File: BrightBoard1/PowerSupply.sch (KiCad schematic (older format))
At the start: 21 parts, among them J2 VIN_JACK, U2 TPS62177DQC

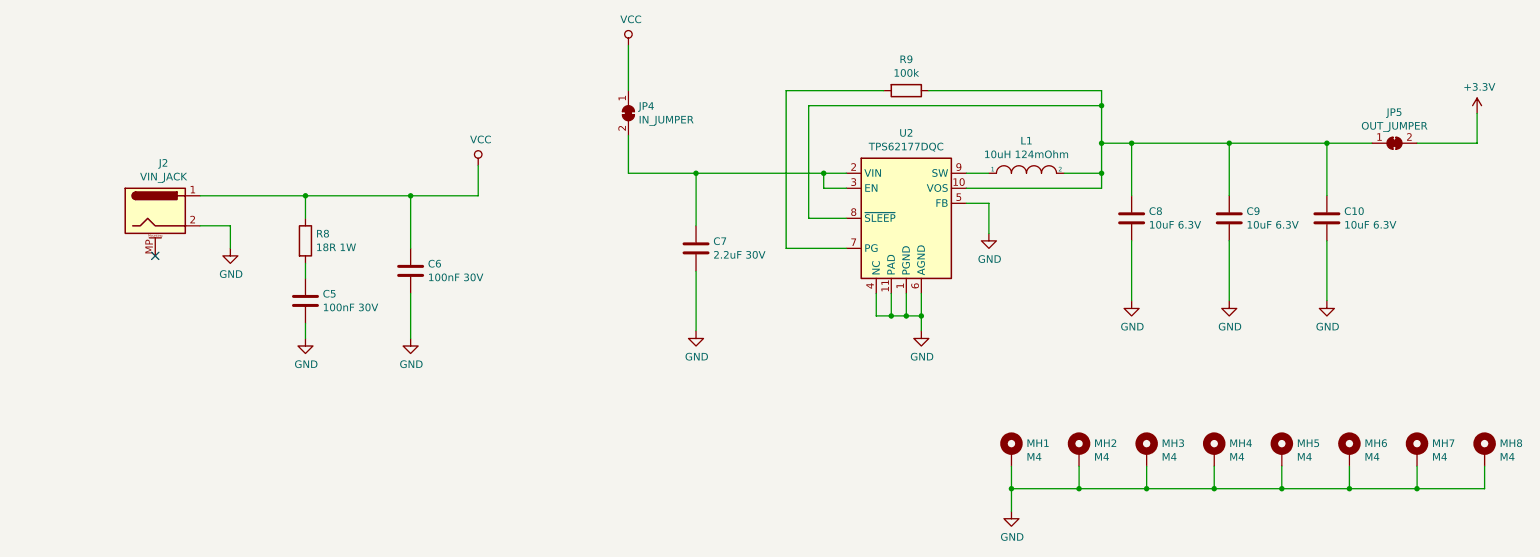
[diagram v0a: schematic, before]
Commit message: Moving over?
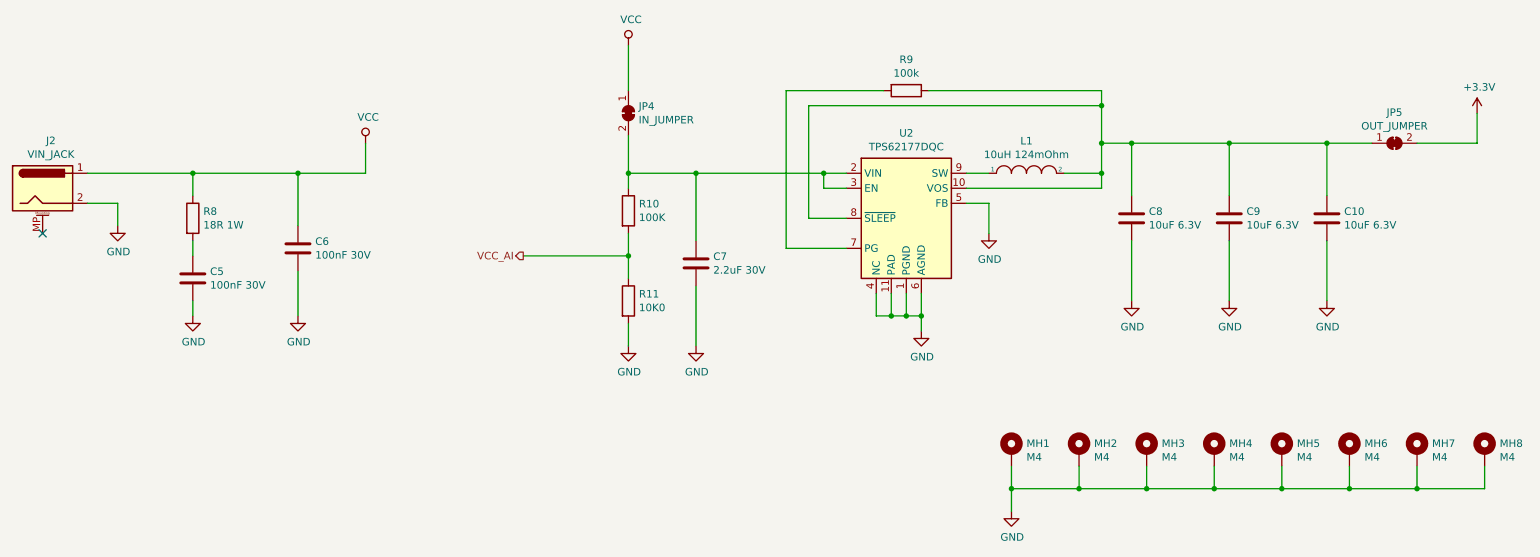
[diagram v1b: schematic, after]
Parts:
- added R10: 100K, Resistor_SMD:R_0805_2012Metric_Pad1.15x1.40mm_HandSolder, symbol Device:R
- added R11: 10K0, Resistor_SMD:R_0805_2012Metric_Pad1.15x1.40mm_HandSolder, symbol Device:R
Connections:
- net GND: now also R11.2
- net at C7.1, JP4.2 (B), U2.2 (VIN)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: now also R10.1
- new net VCC_AI: R10.2, R11.1
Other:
- moved on the sheet: C5, C6, C7, J2, R8
